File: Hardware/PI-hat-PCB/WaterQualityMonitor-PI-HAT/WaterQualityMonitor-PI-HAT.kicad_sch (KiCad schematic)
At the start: 21 parts

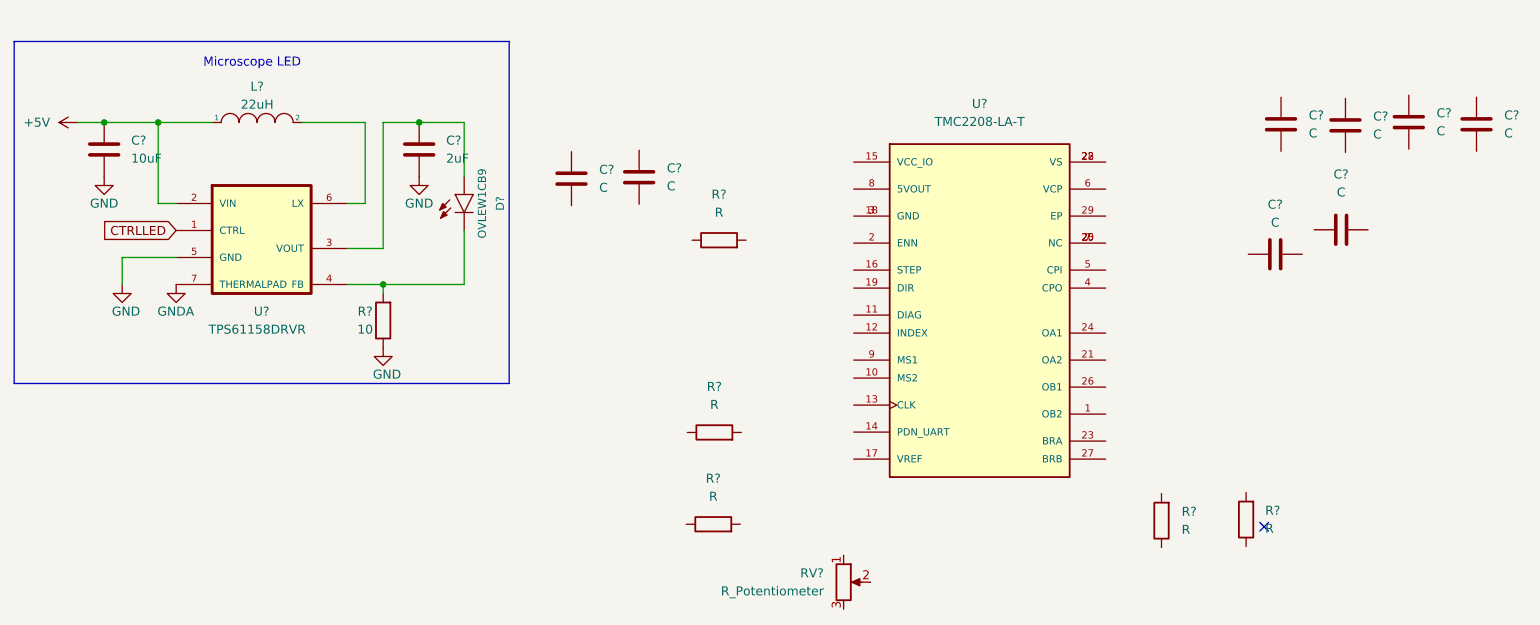
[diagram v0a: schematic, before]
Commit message: worked on stepper motor driver
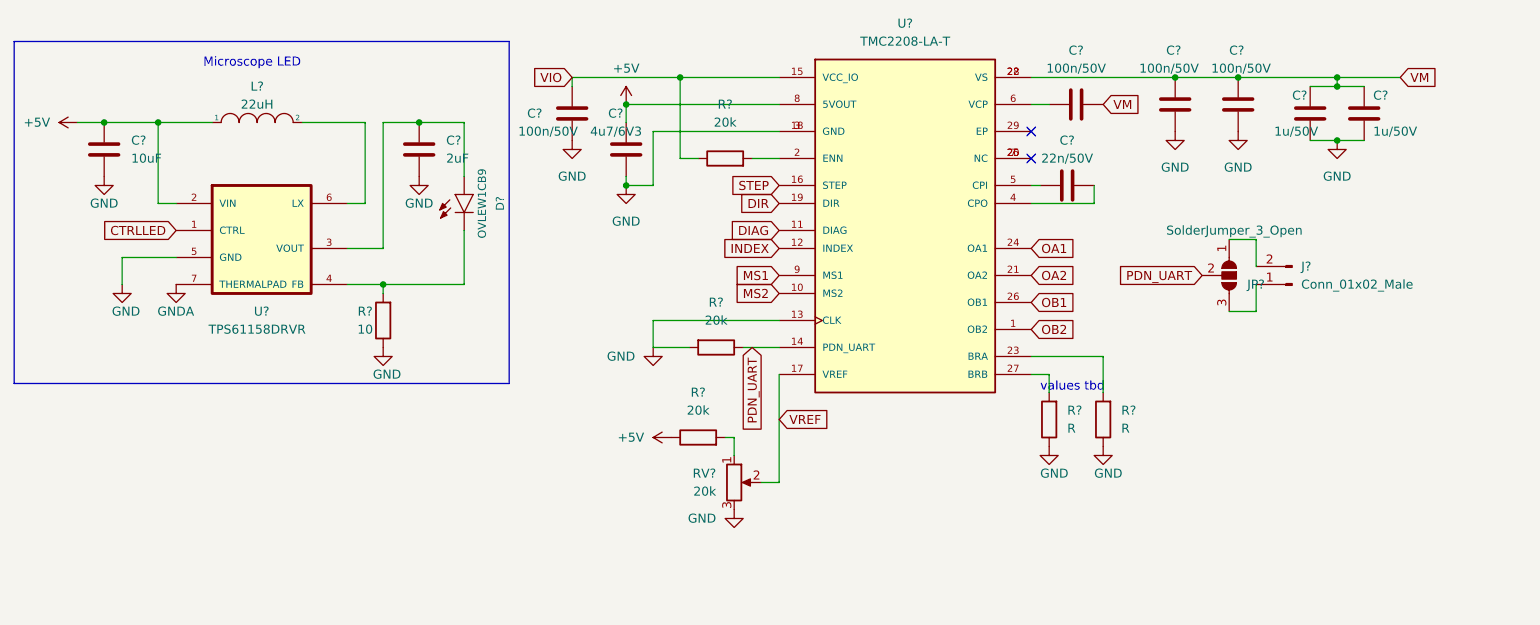
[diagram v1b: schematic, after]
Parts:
- removed R?: R, symbol Device:R
- added J?: Conn_01x02_Male, symbol Connector:Conn_01x02_Male
- added JP?: SolderJumper_3_Open, symbol Jumper:SolderJumper_3_Open
- added R?: 20k, symbol Device:R
- C? (x2): value C -> 1u/50V
- C? (x4): value C -> 100n/50V
- C?: value C -> 4u7/6V3
- C?: value C -> 22n/50V
- R? (x2): value R -> 20k
- RV?: value R_Potentiometer -> 20k
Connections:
- net +5V: now also C?.2, R?.1, U?.8 (5VOUT)
- net GND: now also C?.1, C?.1, C?.1, C?.1, C?.1, C?.1, R?.1, R?.1, RV?.3, U?.13 (CLK), U?.18 (GND), U?.3 (GND), R?.2
- net at RV?.1: now also R?.2
- net VREF: now reaches RV?.2
- net VREF: now also U?.17 (VREF)
- net OB2: now reaches U?.1 (OB2)
- net MS2: now reaches U?.10 (MS2)
- net DIAG: now reaches U?.11 (DIAG)
- net INDEX: now reaches U?.12 (INDEX)
- net PDN_UART: now reaches U?.14 (PDN_UART)
- net PDN_UART: now also JP?.2 (C), R?.1
- net VIO: now reaches U?.15 (VCC_IO)
- net VIO: now also C?.2, R?.1
- net STEP: now reaches U?.16 (STEP)
- net DIR: now reaches U?.19 (DIR)
- net at U?.2 (ENN): now also R?.2
- net OA2: now reaches U?.21 (OA2)
- net VM: now reaches U?.22 (VS), U?.28 (VS)
- net VM: now also C?.2, C?.2, C?.2, C?.2, C?.2
- net at U?.23 (BRA): now also R?.2
- net OA1: now reaches U?.24 (OA1)
- net OB1: now reaches U?.26 (OB1)
- net at U?.27 (BRB): now also R?.2
- net at U?.4 (CPO): now also C?.1
- net at U?.5 (CPI): now also C?.2
- net at U?.6 (VCP): now also C?.1
- net MS1: now reaches U?.9 (MS1)
- new net: J?.2 (Pin_2), JP?.1 (A)
- new net: J?.1 (Pin_1), JP?.3 (B)
- no-connect marks 1 -> 2
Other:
- note added: "values tbd"
- moved on the sheet: C?, R?, RV?, U?
